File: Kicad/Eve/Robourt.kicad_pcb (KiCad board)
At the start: 4 copper layers, 85 x 70 mm, 172 parts, among them IC101 STM32U535RET6, J1 Conn_02x08_Odd_Even, J101 Conn_ST_STDC14, J102 Conn_01x02, J103 Conn_01x02, J108 Conn_01x03, J109 Conn_01x03, J110 Conn_01x02, J115 Conn_02x20_Odd_Even, J201 Conn_01x04, J301 Conn_01x04, J401 Conn_01x04, Q101 NMOS, Q201 SQJ504EP-T1_GE3, Q202 SQJ504EP-T1_GE3, Q203 SQJ504EP-T1_GE3, Q204 SQJ504EP-T1_GE3, Q301 SQJ504EP-T1_GE3, Q302 SQJ504EP-T1_GE3, Q303 SQJ504EP-T1_GE3, Q304 SQJ504EP-T1_GE3, Q401 SQJ504EP-T1_GE3, Q402 SQJ504EP-T1_GE3, Q403 SQJ504EP-T1_GE3, Q404 SQJ504EP-T1_GE3, SW101 SW_Push, SW102 SW_Push, SW103 SW_Push, SW104 SW_Push, U201 TMC2590-TA, U301 TMC2590-TA, U401 TMC2590-TA, U501 BU33SD5WG-TR, U601 LT1076CR-PBF, U701 LT1076CR-PBF, U801 LT1076CR-PBF, Y101 Crystal

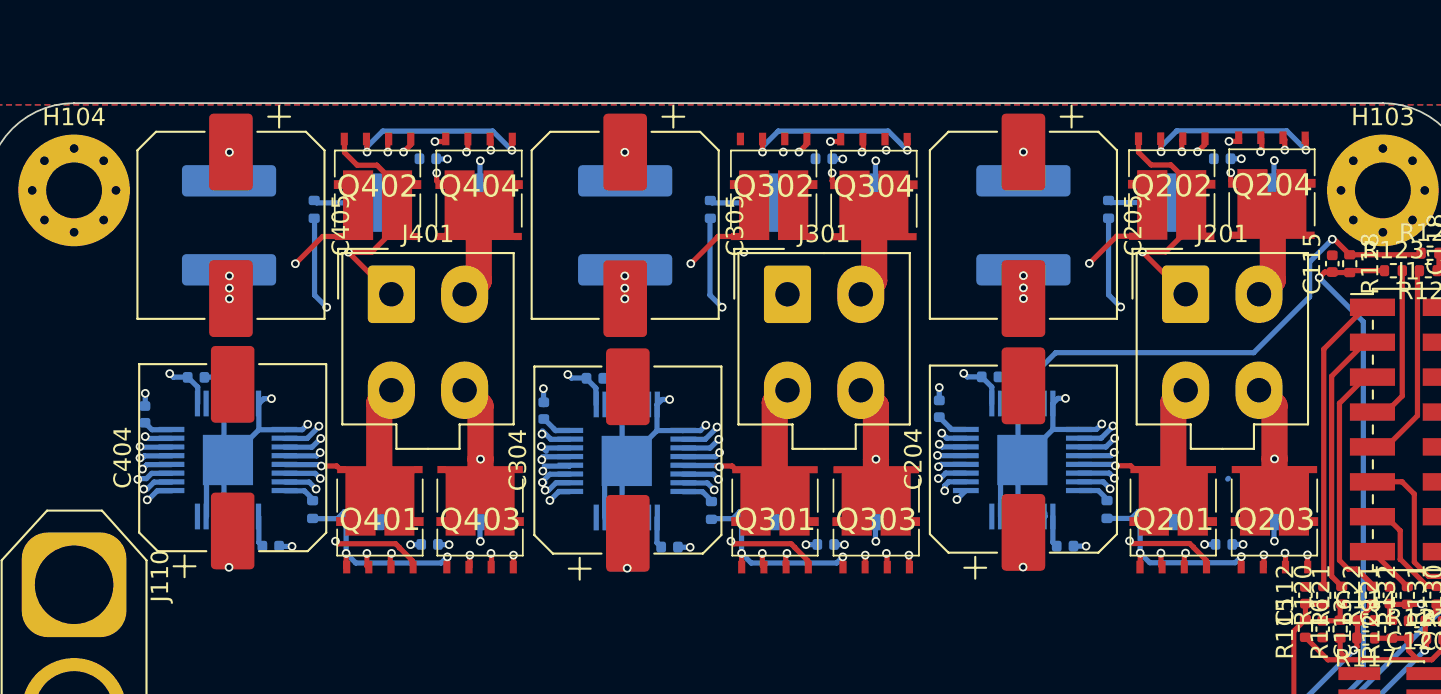
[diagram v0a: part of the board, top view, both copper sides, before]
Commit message: PCB cleaning
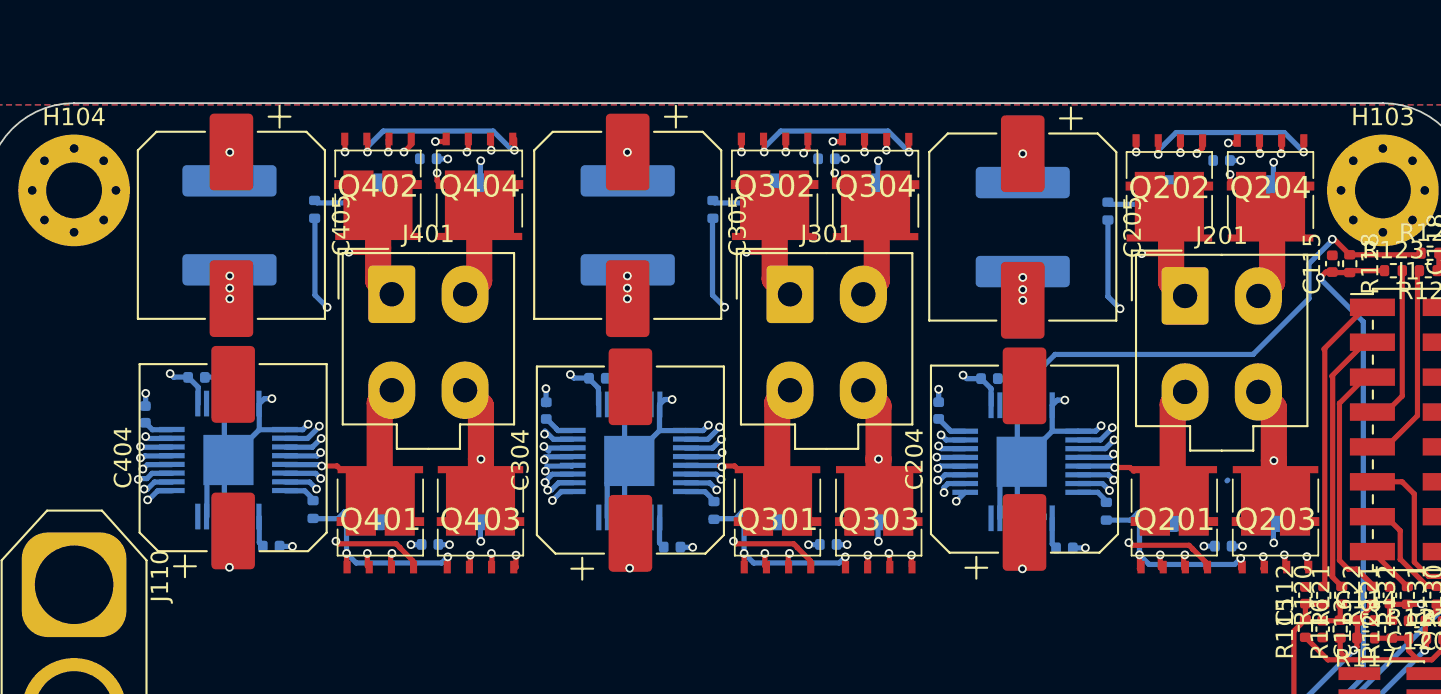
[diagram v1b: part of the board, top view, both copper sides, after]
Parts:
- moved Q204 0.17 mm to (94.6, 22.7)
- moved Q202 0.17 mm to (88.8, 22.7)
- moved Q303 0.15 mm to (72.1, 45.8)
- moved R301 0.15 mm to (69.1, 42.7)
- moved R302 0.15 mm to (69.1, 25.6)
- moved C303 0.15 mm to (57.7, 26.9)
- moved C305 0.15 mm to (57.7, 26.9)
- moved R304 0.15 mm to (62.6, 26.0)
- moved U301 0.15 mm to (57.8, 40.4)
- moved C301 0.14 mm to (69.1, 23.1)
- moved C302 0.14 mm to (69.2, 45.2)
- moved C304 0.14 mm to (57.9, 40.4)
- moved C306 0.14 mm to (53.1, 37.5)
- moved C307 0.14 mm to (56.0, 35.7)
- moved C308 0.14 mm to (60.3, 45.3)
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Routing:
- net /driver_stepper1/B1: track 19.2 -> 26.6 mm
- net /driver_stepper2/B1: track 33.2 -> 26.7 mm
- net /driver_stepper2/HB1: track 18.2 -> 23.4 mm
- net /driver_stepper1/HB1: track 18.1 -> 23.2 mm
- net /driver_stepper/HB1: track 17.9 -> 23.0 mm
- net /driver_stepper/B1: track 32.9 -> 29.7 mm
- net /driver_stepper1/LB1: track 34.3 -> 35.1 mm
- net /driver_stepper1/LB2: track 31.3 -> 32.0 mm
